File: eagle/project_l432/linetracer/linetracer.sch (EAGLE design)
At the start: 24 parts, among them IC1 TA4805S, Q1 IRFU5505PBF, Q2 RPR-220, Q3 RPR-220, Q4 RPR-220, U1 TA8428K(O,S), U2 TA8428K(O,S)

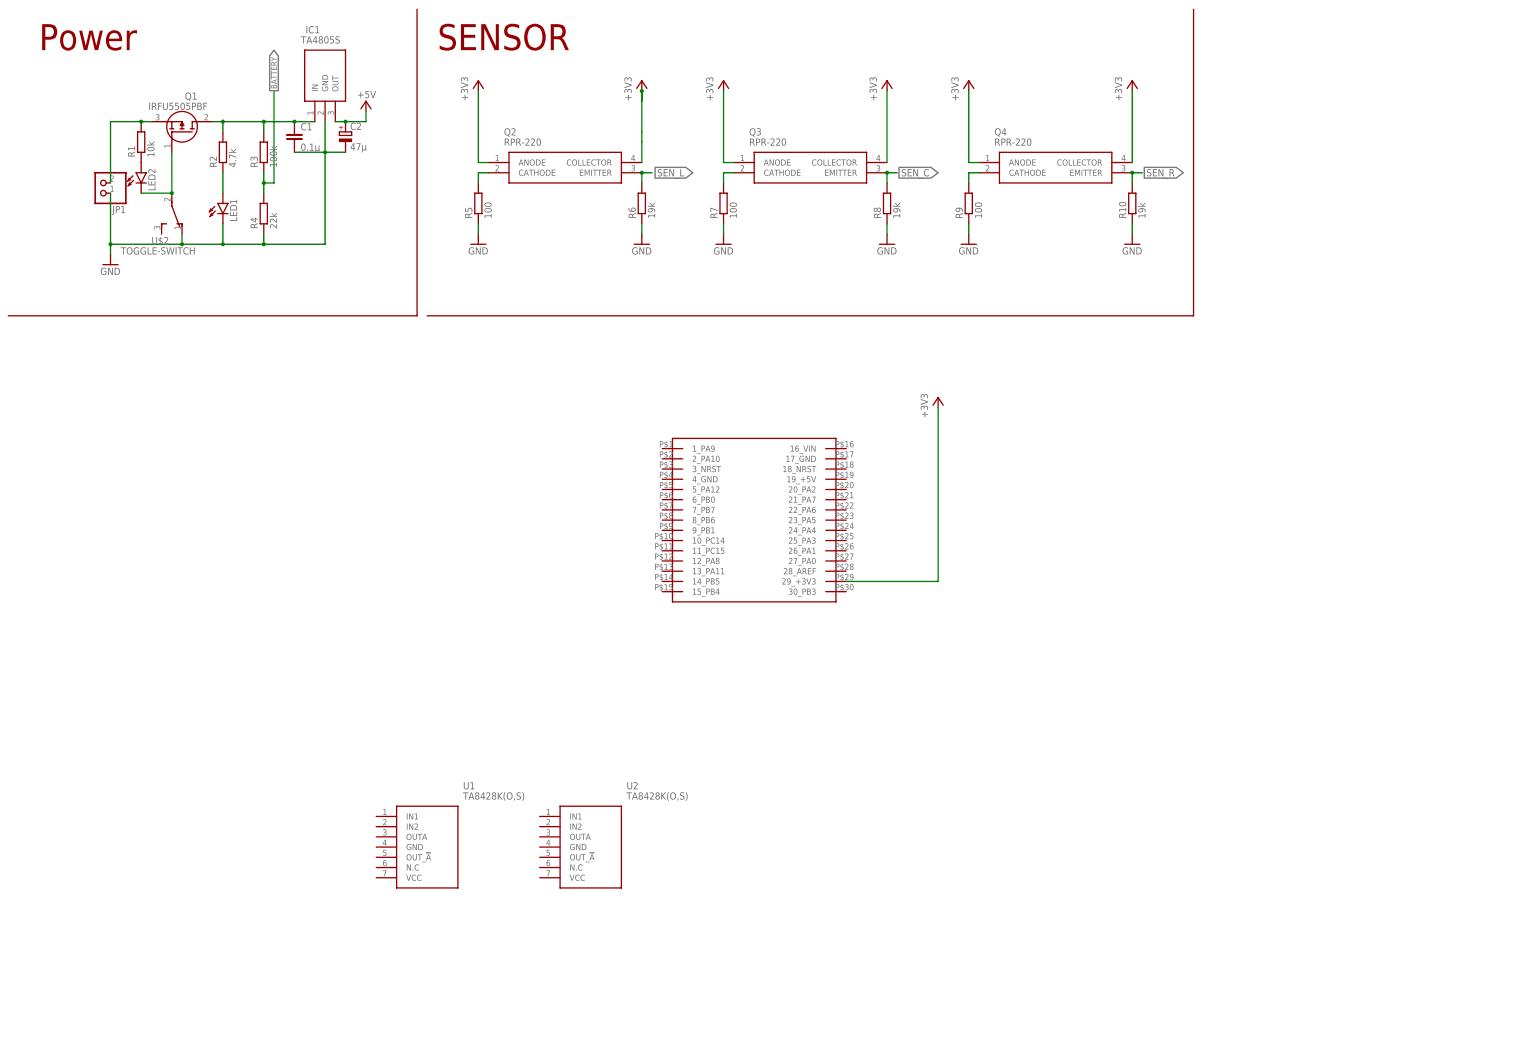
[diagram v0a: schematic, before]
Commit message: schematic
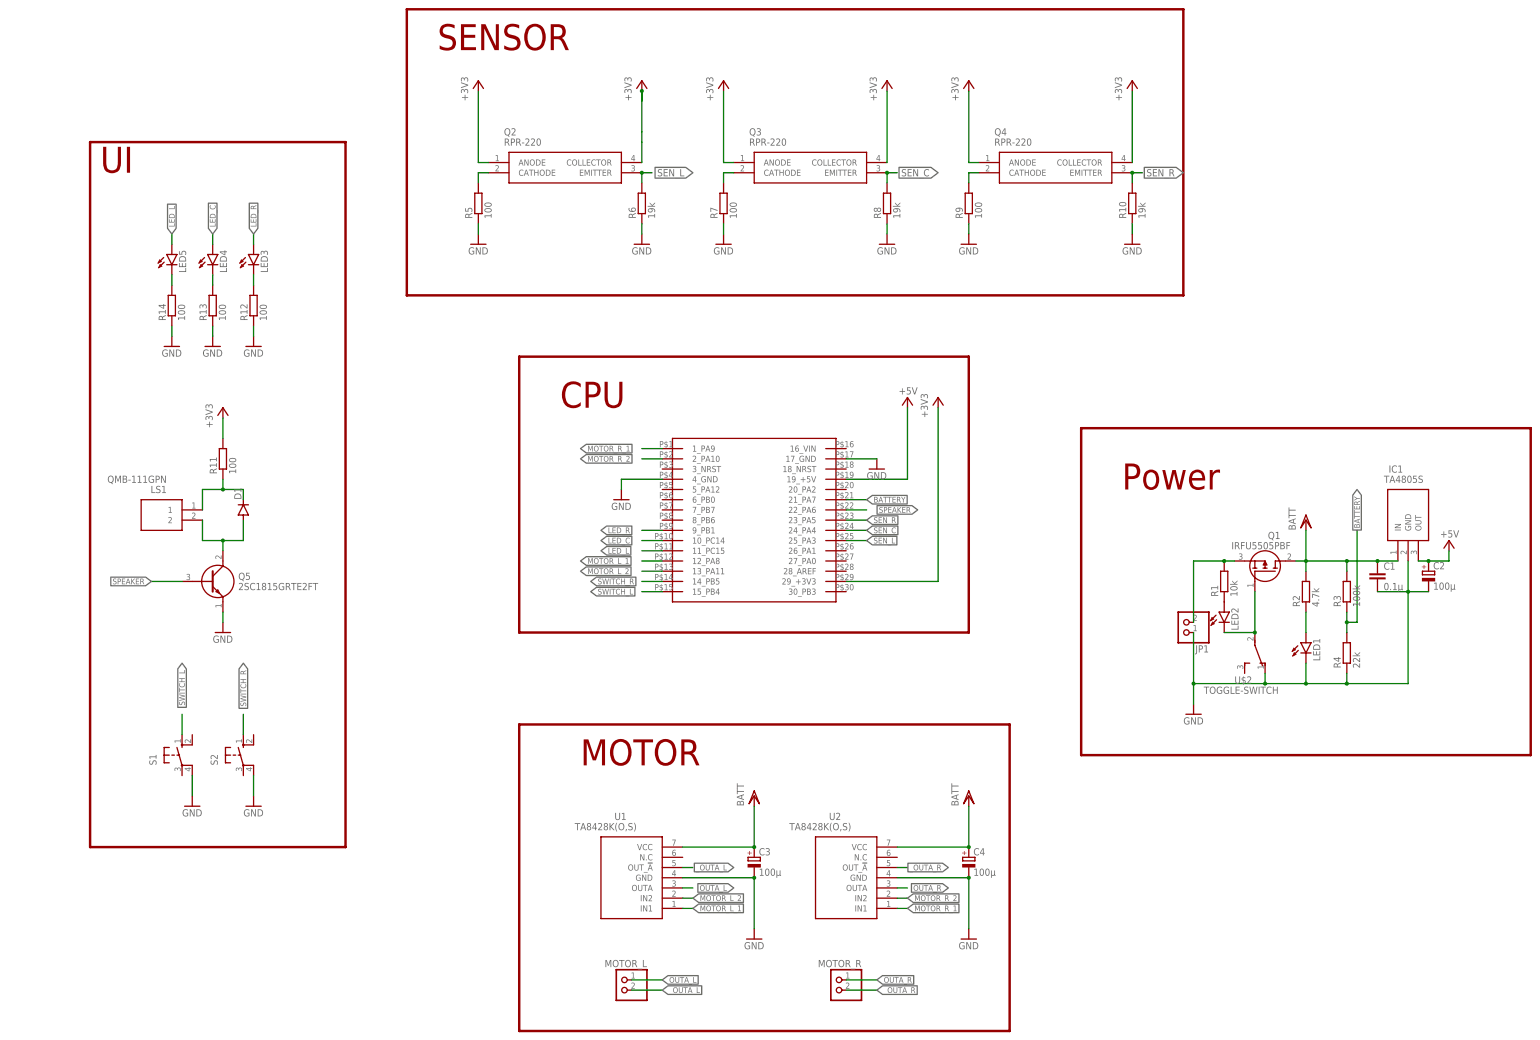
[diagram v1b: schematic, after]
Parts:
- added C3, C4: 100μ, rcl:CPOL-EUE2.5-7
- added D1: (no value), diode:DIODE-DO07
- added LED3, LED4, LED5: (no value), led:LED3MM
- added LS1: QMB-111GPN, QMB-111GPN:QMB-111GPN
- added MOTOR_L, MOTOR_R: (no value), pinhead:PINHD-1X2
- added Q5: 2SC1815GRTE2FT, 2SC1815GRTE2FT:2SC1815GRTE2FT
- added R11, R12, R13, R14: 100, rcl:R-EU_0204/2V
- added S1, S2: (no value), switch-omron:10-XX
- C2: value 47μ -> 100μ; device rcl:CPOL-EUE5-10.5 -> rcl:CPOL-EUE2.5-7
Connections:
- new net BATT: C1.1, C3.+, C4.+, IC1.IN, Q1.D, R2.2, R3.2, U1.VCC, U2.VCC
- new net LED_C: LED4.A, U$1.10_PC14
- new net LED_L: LED5.A, U$1.11_PC15
- new net LED_R: LED3.A, U$1.9_PB1
- new net MOTOR_L_1: U$1.12_PA8, U1.IN1
- new net MOTOR_L_2: U$1.13_PA11, U1.IN2
- new net MOTOR_R_1: U$1.1_PA9, U2.IN1
- new net MOTOR_R_2: U$1.2_PA10, U2.IN2
- new net N$10: LED3.C, R12.2
- new net N$11: LED4.C, R13.2
- new net N$12: LED5.C, R14.2
- new net N$9: D1.A, LS1.2, Q5.C
- new net OUTA_L: MOTOR_L.1, U1.OUTA
- new net OUTA_R: MOTOR_R.1, U2.OUTA
- new net SPEAKER: Q5.B, U$1.22_PA6
- new net SWITCH_L: S1.S, U$1.15_PB4
- new net SWITCH_R: S2.S, U$1.14_PB5
- new net _OUTA_L: MOTOR_L.2, U1.OUT_!A
- new net _OUTA_R: MOTOR_R.2, U2.OUT_!A
- net +3V3: now also R11.2
- net +5V: now also U$1.19_+5V
- net BATTERY: now also U$1.21_PA7
- net GND: now also C3.-, C4.-, Q5.E, R12.1, R13.1, R14.1, S1.P1, S2.P1, U$1.17_GND, U$1.4_GND, U1.GND, U2.GND
- net N$4: now also D1.C, LS1.1, R11.1; no longer C1.1, IC1.IN, Q1.D, R2.2, R3.2
- net SEN_C: now also U$1.24_PA4
- net SEN_L: now also U$1.25_PA3
- net SEN_R: now also U$1.23_PA5
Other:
- note added: "CPU"
- note added: "MOTOR"
- note added: "UI"
- moved on the sheet: C1, C2, IC1, JP1, LED1, LED2, Q1, R1, R2, R3, R4, U$2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
